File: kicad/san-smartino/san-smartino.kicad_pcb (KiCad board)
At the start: 2 copper layers, 80.3 x 80.3 mm, 53 parts, among them J1 GND CTS VBUS RX TX DTR, J2 SDA SCL -3V3 GND, J3 Conn_01x07_Male, SW1 Reset, SW2 Flash, U1 BQ27441DRZR-G1A, U2 ESP-12E, U3 LTC3440

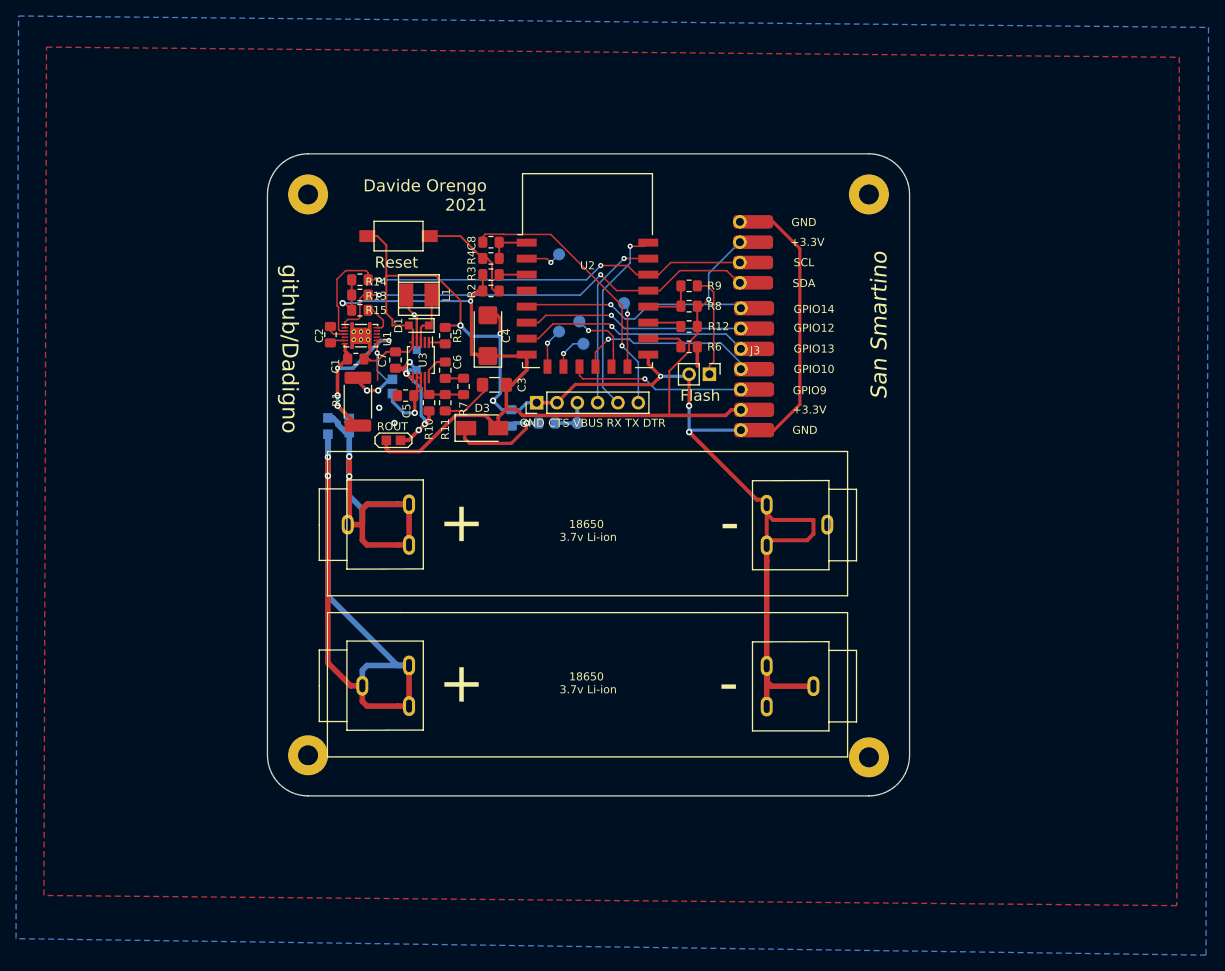
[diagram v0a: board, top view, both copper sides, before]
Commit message: updated board
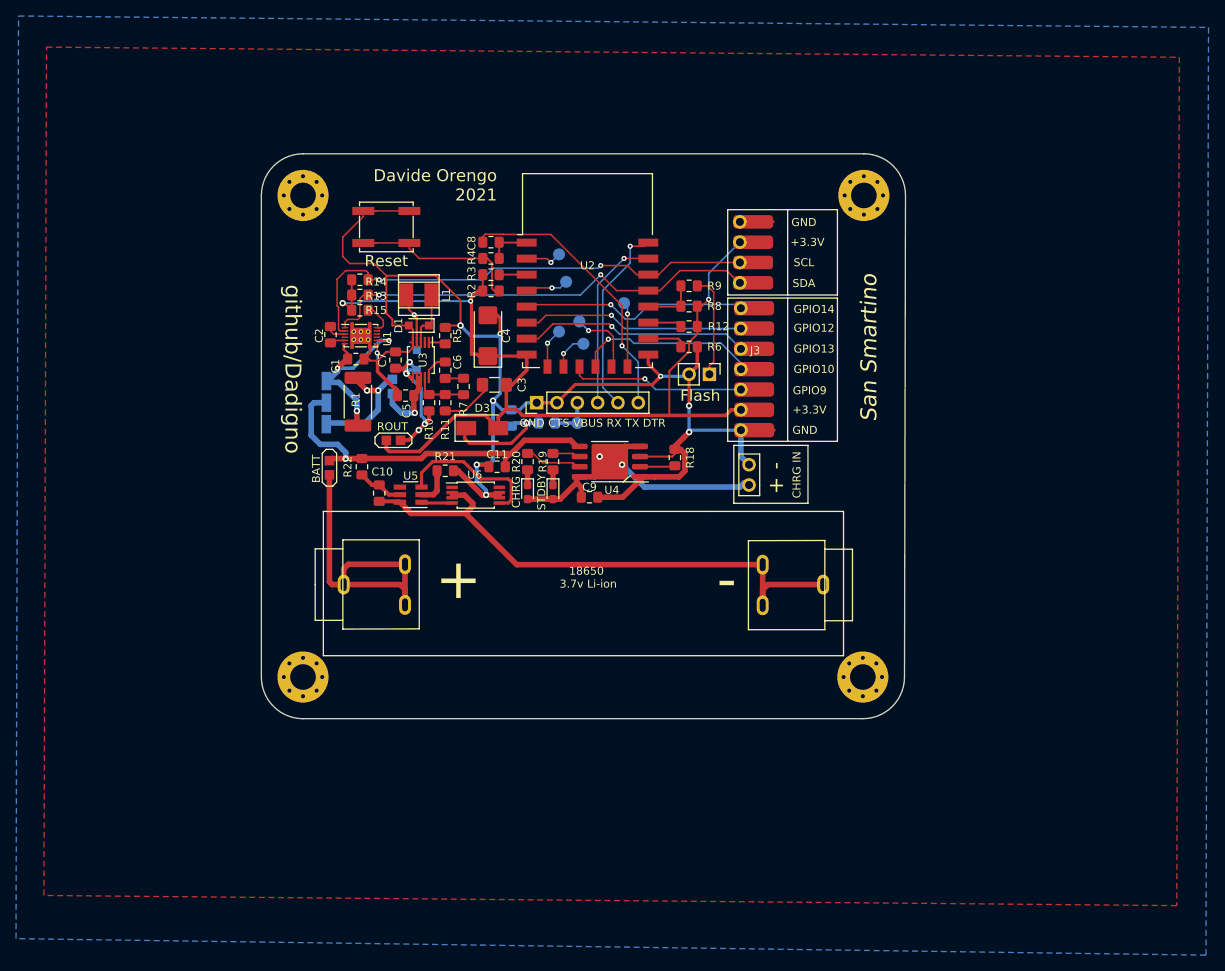
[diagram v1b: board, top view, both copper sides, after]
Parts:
- removed BT2: 2.45v-4.5v, san-smartino:18650-battery-metal-clips
- removed REF** (x4): MountingHole_2.5mm_Pad, MountingHole:MountingHole_2.5mm_Pad
- added C10: 100nF, Capacitor_SMD:C_0805_2012Metric_Pad1.15x1.40mm_HandSolder, F.Cu at (82.5, 64.0)
- added C11: 10uF, Capacitor_SMD:C_0805_2012Metric_Pad1.15x1.40mm_HandSolder, F.Cu at (97.3, 60.7)
- added C9: 0.1uF, Capacitor_SMD:C_0805_2012Metric_Pad1.15x1.40mm_HandSolder, F.Cu at (108.8, 64.5)
- added D4: STDBY, LED_SMD:LED_0603_1608Metric_Pad1.05x0.95mm_HandSolder, F.Cu at (104.3, 63.9)
- added D5: CHRG, LED_SMD:LED_0603_1608Metric_Pad1.05x0.95mm_HandSolder, F.Cu at (101.1, 63.9)
- added H1: MountingHole, MountingHole:MountingHole_3.2mm_M3_Pad_Via, F.Cu at (73.0, 26.8)
- added H2: MountingHole, MountingHole:MountingHole_3.2mm_M3_Pad_Via, F.Cu at (73.0, 87.0)
- added H3: MountingHole, MountingHole:MountingHole_3.2mm_M3_Pad_Via, F.Cu at (143.1, 26.8)
- added H4: MountingHole, MountingHole:MountingHole_3.2mm_M3_Pad_Via, F.Cu at (143.0, 87.0)
- added J4: CHRG IN, Connector_PinHeader_2.54mm:PinHeader_1x02_P2.54mm_Vertical, F.Cu at (128.8, 63.0)
- added J5: PW-SEL, Connector_PinHeader_2.54mm:PinHeader_1x03_P2.54mm_Vertical, B.Cu at (75.9, 55.2)
- added R18: 1.2k, Resistor_SMD:R_0805_2012Metric_Pad1.15x1.40mm_HandSolder, F.Cu at (119.5, 59.6)
- added R19: 1k, Resistor_SMD:R_0805_2012Metric_Pad1.15x1.40mm_HandSolder, F.Cu at (104.3, 60.1)
- added R20: 1k, Resistor_SMD:R_0805_2012Metric_Pad1.15x1.40mm_HandSolder, F.Cu at (101.1, 60.1)
- added R21: 1k, Resistor_SMD:R_0805_2012Metric_Pad1.15x1.40mm_HandSolder, F.Cu at (90.8, 61.2)
- added R22: 100R, Resistor_SMD:R_0805_2012Metric_Pad1.15x1.40mm_HandSolder, F.Cu at (80.4, 60.7)
- added U4: TP4056, Package_SO:SOP-8-1EP_4.57x4.57mm_P1.27mm_EP4.57x4.45mm, F.Cu at (111.4, 60.1)
- added U5: DW01, Package_TO_SOT_SMD:SOT-23-6_Handsoldering, F.Cu at (86.5, 64.2)
- added U6: FS8205A, Package_SO:TSSOP-8_4.4x3mm_P0.65mm, F.Cu at (94.6, 64.3)
- SW1: footprint Button_Switch_SMD:SW_SPST_CK_RS282G05A3 -> Button_Switch_SMD:SW_SPST_EVQP0
- TP10: value BATT_2 -> Wake; footprint TestPoint:TestPoint_2Pads_Pitch2.54mm_Drill0.8mm -> TestPoint:TestPoint_Pad_D1.5mm
- TP9: value BATT_1 -> BATT; moved to F.Cu
- moved TP10 35.5 mm to (105.9, 37.6), turned to 0 degrees
- moved BT1 7.51 mm to (74.3, 75.4)
- moved TP9 5.82 mm to (76.3, 62.1)
- moved SW1 1.90 mm to (83.4, 30.7)
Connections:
- net +BATT renamed VCC
- net /BIN renamed Net-(U1-Pad10)
- BT1 pad 2: -BATT -> BATT-
- C1 pad 1: Net-(C1-Pad1) -> FUEL-GAUGE
- C1 pad 2: -BATT -> IN-
- C2 pad 2: -BATT -> IN-
- C3 pad 2: -BATT -> IN-
- C4 pad 2: -BATT -> IN-
- C5 pad 2: -BATT -> IN-
- C7 pad 2: -BATT -> IN-
- D1 pad 2: -BATT -> IN-
- J1 pad 1: -BATT -> IN-
- J1 pad 2: -BATT -> IN-
- J2 pad 1: -BATT -> IN-
- J3 pad 7: -BATT -> IN-
- R1 pad 1: Net-(C1-Pad1) -> FUEL-GAUGE
- R11 pad 2: -BATT -> IN-
- R17 pad 2: -BATT -> IN-
- R5 pad 2: -BATT -> IN-
- R6 pad 2: -BATT -> IN-
- SW1 pad 1: -BATT -> IN-
- SW2 pad 2: -BATT -> IN-
- TP10 pad 1: Net-(BT2-Pad1) -> /WAKE
- TP9 pad 2: Net-(C1-Pad1) -> BATT+
- U1 pad 13: -BATT -> IN-
- U1 pad 3: -BATT -> IN-
- U1 pad 6: Net-(C1-Pad1) -> FUEL-GAUGE
- U1 pad 8: Net-(C1-Pad1) -> FUEL-GAUGE
- U2 pad 15: -BATT -> IN-
- U2 pad 4: (no net) -> /WAKE
- U3 pad 5: -BATT -> IN-
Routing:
- net -BATT: track 224.1 -> 0.00 mm, vias 8 -> 0
- net IN-: track 0.00 -> 202.2 mm, vias 0 -> 8
- net Net-(BT2-Pad1): track 91.5 -> 0.00 mm, vias 2 -> 0
- net BATT-: track 0.00 -> 71.3 mm
- net BATT+: track 0.00 -> 46.0 mm, vias 0 -> 1
- net IN+: track 0.00 -> 40.1 mm, vias 0 -> 2
- net Net-(C1-Pad1): track 25.6 -> 0.00 mm, vias 4 -> 0
- net FUEL-GAUGE: track 0.00 -> 23.9 mm, vias 0 -> 3
- net Net-(U5-Pad3): track 0.00 -> 18.5 mm
- net Net-(BT1-Pad1): track 53.0 -> 40.1 mm, vias 2 -> 0
- net VCC: track 12.0 -> 21.6 mm
- net Net-(R2-Pad2): track 13.4 -> 21.7 mm
- net Net-(R20-Pad2): track 0.00 -> 6.82 mm
- net Net-(C10-Pad1): track 0.00 -> 5.79 mm
- net /WAKE: track 0.00 -> 5.39 mm, vias 0 -> 1
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- added copper zone on B.Cu, net IN-
- added copper zone on F.Cu, net IN-
- removed copper zone on B.Cu, net -BATT
- removed copper zone on F.Cu, net -BATT
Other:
- board size 80.3 x 80.3 mm -> 80.5 x 70.6 mm
